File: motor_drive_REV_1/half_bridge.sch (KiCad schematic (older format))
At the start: 5 parts, among them Q1 nmos, Q2 nmos

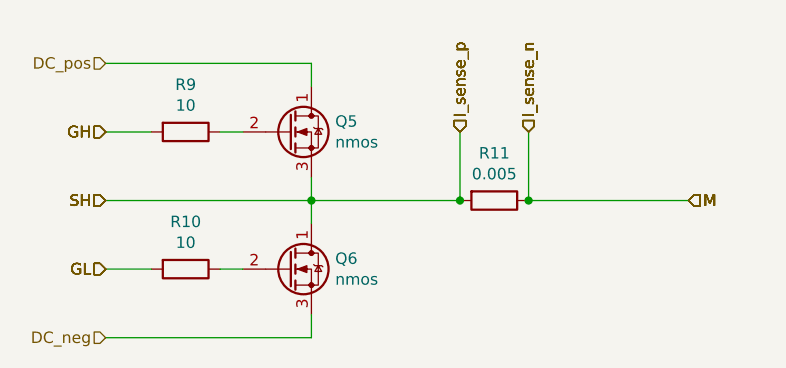
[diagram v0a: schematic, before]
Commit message: started layout
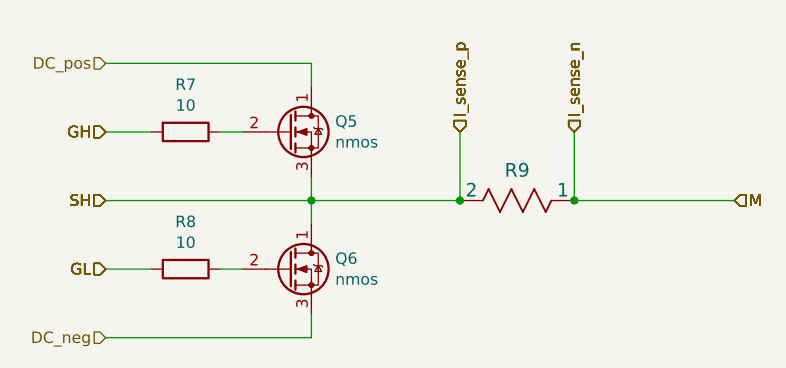
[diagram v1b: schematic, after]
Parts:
- removed R5: 0.005, motor_drive_footprints:C_0603_1608Metric, symbol motor_drive:R
- added R6: WSL20101L000FEA18, motor_drive_footprints:WSL20101L000FEA18, symbol motor_drive:WSL20101L000FEA18
- renumbered R3 to R1, R4 to R2
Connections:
- net I_sense_n: now also R6.1
- net I_sense_p: now also R6.2
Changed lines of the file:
@@
 $Descr A4 11693 8268
 encoding utf-8
-Sheet 4 14
+Sheet 4 16
 Title ""
 Date ""
@@
 Text HLabel 5750 3400 1    50   Input ~ 0
 I_sense_p
-Text HLabel 6050 3400 1    50   Input ~ 0
+Text HLabel 6250 3400 1    50   Input ~ 0
 I_sense_n
 Text HLabel 4200 4000 0    50   Input ~ 0
@@
 Wire Wire Line
 	4200 3700 5100 3700
-Text HLabel 6750 3700 2    50   Input ~ 0
+Text HLabel 6950 3700 2    50   Input ~ 0
 M
 Text HLabel 5750 3400 1    50   Input ~ 0
 I_sense_p
-Text HLabel 6050 3400 1    50   Input ~ 0
+Text HLabel 6250 3400 1    50   Input ~ 0
 I_sense_n
 Text HLabel 4200 4000 0    50   Input ~ 0
@@
 Text HLabel 4200 3700 0    50   Input ~ 0
 SH
-Text HLabel 6750 3700 2    50   Input ~ 0
+Text HLabel 6950 3700 2    50   Input ~ 0
 M
 Text HLabel 5750 3400 1    50   Input ~ 0
 I_sense_p
-Text HLabel 6050 3400 1    50   Input ~ 0
+Text HLabel 6250 3400 1    50   Input ~ 0
 I_sense_n
 Text HLabel 4200 4000 0    50   Input ~ 0
@@
 Text HLabel 4200 3700 0    50   Input ~ 0
 SH
-Text HLabel 6750 3700 2    50   Input ~ 0
+Text HLabel 6950 3700 2    50   Input ~ 0
 M
 Text HLabel 5750 3400 1    50   Input ~ 0
 I_sense_p
-Text HLabel 6050 3400 1    50   Input ~ 0
+Text HLabel 6250 3400 1    50   Input ~ 0
 I_sense_n
 Text HLabel 4200 4000 0    50   Input ~ 0
@@
 Text HLabel 4200 3700 0    50   Input ~ 0
 SH
-Text HLabel 6750 3700 2    50   Input ~ 0
+Text HLabel 6950 3700 2    50   Input ~ 0
 M
 $Comp
@@
 $EndComp
 $Comp
-L motor_drive:R R4
+L motor_drive:R R2
 U 1 1 5E27A2EF
 P 4550 4000
-AR Path="/5E257703/5E27A2EF" Ref="R4"  Part="1"
-AR Path="/5E26944C/5E27A2EF" Ref="R7"  Part="1"
-AR Path="/5E26B60E/5E27A2EF" Ref="R10"  Part="1"
-F 0 "R10" V 4343 4000 50  0000 C CNN
+AR Path="/5E257703/5E27A2EF" Ref="R2"  Part="1"
+AR Path="/5E26944C/5E27A2EF" Ref="R5"  Part="1"
+AR Path="/5E26B60E/5E27A2EF" Ref="R8"  Part="1"
+F 0 "R8" V 4343 4000 50  0000 C CNN
 F 1 "10" V 4434 4000 50  0000 C CNN
 F 2 "motor_drive_footprints:C_0603_1608Metric" V 4480 4000 50  0001 C CNN
@@
 $EndComp
 $Comp
-L motor_drive:R R3
+L motor_drive:R R1
 U 1 1 5E27D5F7
 P 4550 3400
-AR Path="/5E257703/5E27D5F7" Ref="R3"  Part="1"
-AR Path="/5E26944C/5E27D5F7" Ref="R6"  Part="1"
-AR Path="/5E26B60E/5E27D5F7" Ref="R9"  Part="1"
-F 0 "R9" V 4343 3400 50  0000 C CNN
+AR Path="/5E257703/5E27D5F7" Ref="R1"  Part="1"
+AR Path="/5E26944C/5E27D5F7" Ref="R4"  Part="1"
+AR Path="/5E26B60E/5E27D5F7" Ref="R7"  Part="1"
+F 0 "R7" V 4343 3400 50  0000 C CNN
 F 1 "10" V 4434 3400 50  0000 C CNN
 F 2 "motor_drive_footprints:C_0603_1608Metric" V 4480 3400 50  0001 C CNN
@@
 	4700 4000 4800 4000
 Wire Wire Line
-	6050 3700 6750 3700
+	6250 3700 6950 3700
 Text HLabel 4200 4300 0    50   Input ~ 0
 DC_neg
@@
 Wire Wire Line
 	5100 4300 5100 4200
-$Comp
-L motor_drive:R R5
-U 1 1 5E35BEDA
-P 5900 3700
-AR Path="/5E257703/5E35BEDA" Ref="R5"  Part="1"
-AR Path="/5E26944C/5E35BEDA" Ref="R8"  Part="1"
-AR Path="/5E26B60E/5E35BEDA" Ref="R11"  Part="1"
-F 0 "R11" V 5693 3700 50  0000 C CNN
-F 1 "0.005" V 5784 3700 50  0000 C CNN
-F 2 "motor_drive_footprints:C_0603_1608Metric" V 5830 3700 50  0001 C CNN
-F 3 "~" H 5900 3700 50  0001 C CNN
-	1    5900 3700
-	0    1    1    0
-$EndComp
 Wire Wire Line
 	5100 3700 5750 3700
 Wire Wire Line
 	5750 3400 5750 3700
-Connection ~ 5750 3700
 Wire Wire Line
-	6050 3400 6050 3700
-Connection ~ 6050 3700
+	6250 3400 6250 3700
 Wire Wire Line
 	5100 3700 5100 3600
@@
 Wire Wire Line
 	4200 4300 5100 4300
+$Comp
+L motor_drive:WSL20101L000FEA18 R6
+U 1 1 5E424CCF
+P 5750 3700
+AR Path="/5E26944C/5E424CCF" Ref="R6"  Part="1"
+AR Path="/5E257703/5E424CCF" Ref="R3"  Part="1"
+AR Path="/5E26B60E/5E424CCF" Ref="R9"  Part="1"
+F 0 "R9" H 6000 3832 60  0000 C CNN
+F 1 "WSL20101L000FEA18" H 6000 3832 60  0001 C CNN
+F 2 "motor_drive_footprints:WSL20101L000FEA18" H 6000 3365 60  0001 C CNN
+F 3 "" H 5750 3700 60  0000 C CNN
+	1    5750 3700
+	1    0    0    -1
+$EndComp
+Connection ~ 5750 3700
+Connection ~ 6250 3700
 $EndSCHEMATC
